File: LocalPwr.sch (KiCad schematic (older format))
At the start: 27 parts, among them U10 TLV702vvDBV, U8 AOZ1282, U9 LM7705

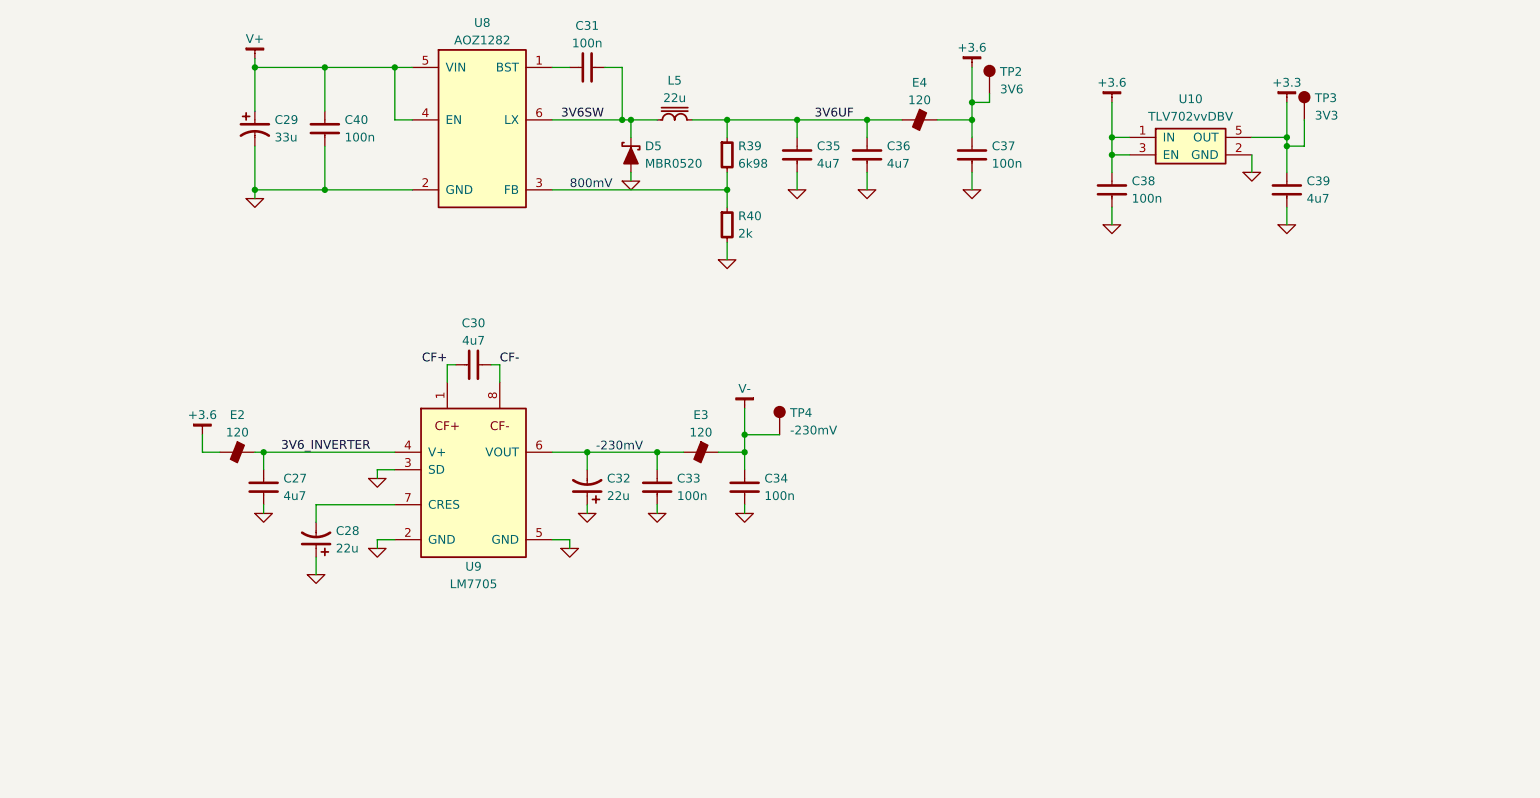
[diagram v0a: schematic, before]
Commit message: First working version
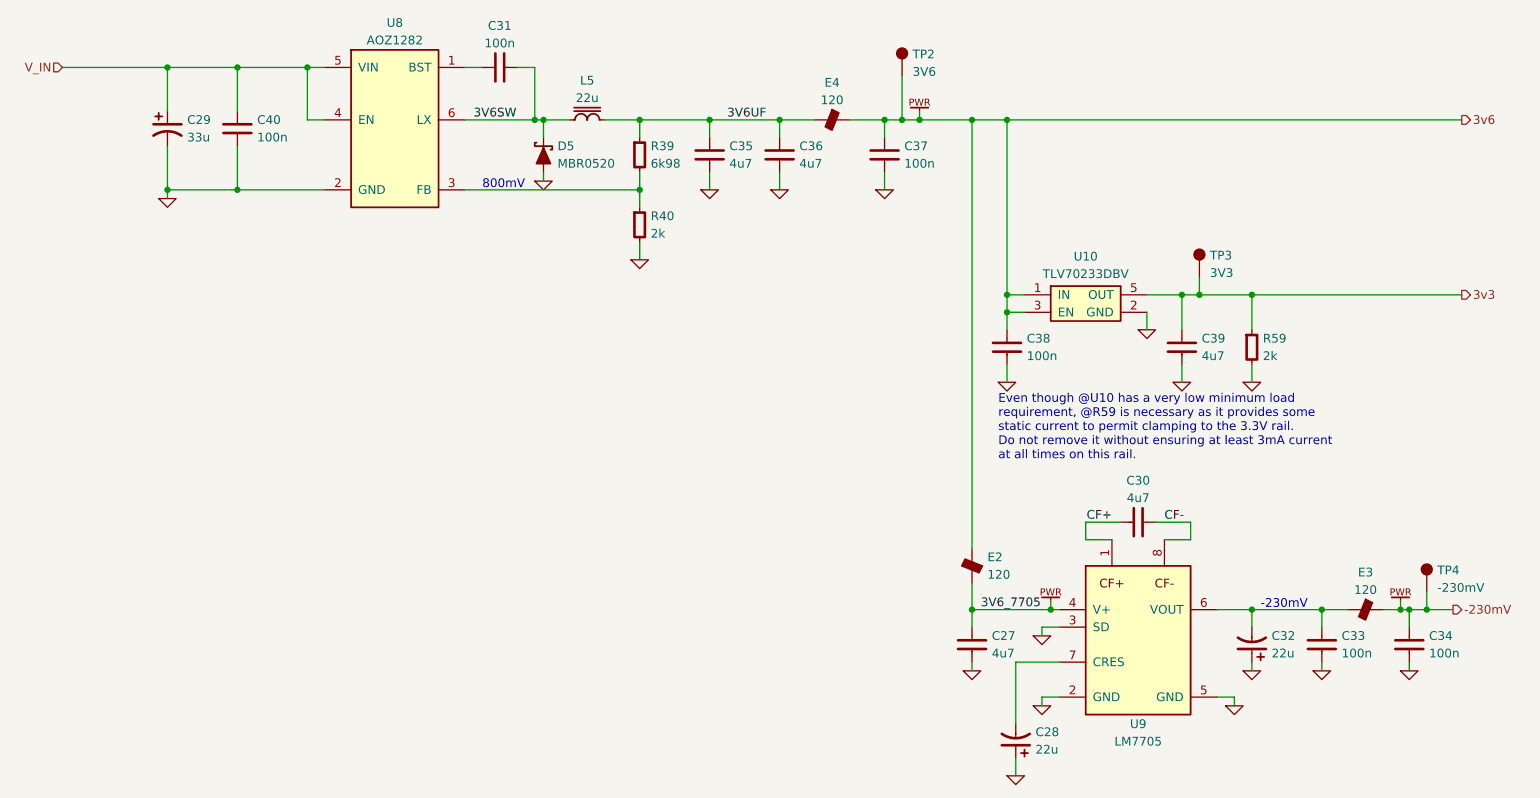
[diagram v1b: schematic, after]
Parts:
- added R59: 2k, IPC7351-Nominal:RESC1608X50, symbol R-0603
- U10: value TLV702vvDBV -> TLV70233DBV; BOM IC TI TLV702vvDBV -> IC TI TLV70233DBV
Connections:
- net GND: now also R59.2
- net +3.3 renamed 3v3
- net 3v3: now also R59.1
- net +3.6 renamed 3v6
- net 3V6_INVERTER renamed 3V6_7705
- net V+ renamed V_IN
- net V- renamed -230mV
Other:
- note added: "Even though @U10 has a very low minimum load\nrequirement, @R59 is necessary as it provides some\nstatic current to permit clamping to the 3.3V rail.\nDo not remove it without ensuring at least 3mA current\nat all times on this rail."
- moved on the sheet: C27, C28, C29, C30, C31, C32, C33, C34, C35, C36, C37, C38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
